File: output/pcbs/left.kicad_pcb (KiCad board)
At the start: 2 copper layers, 143.6 x 118.9 mm, 72 parts

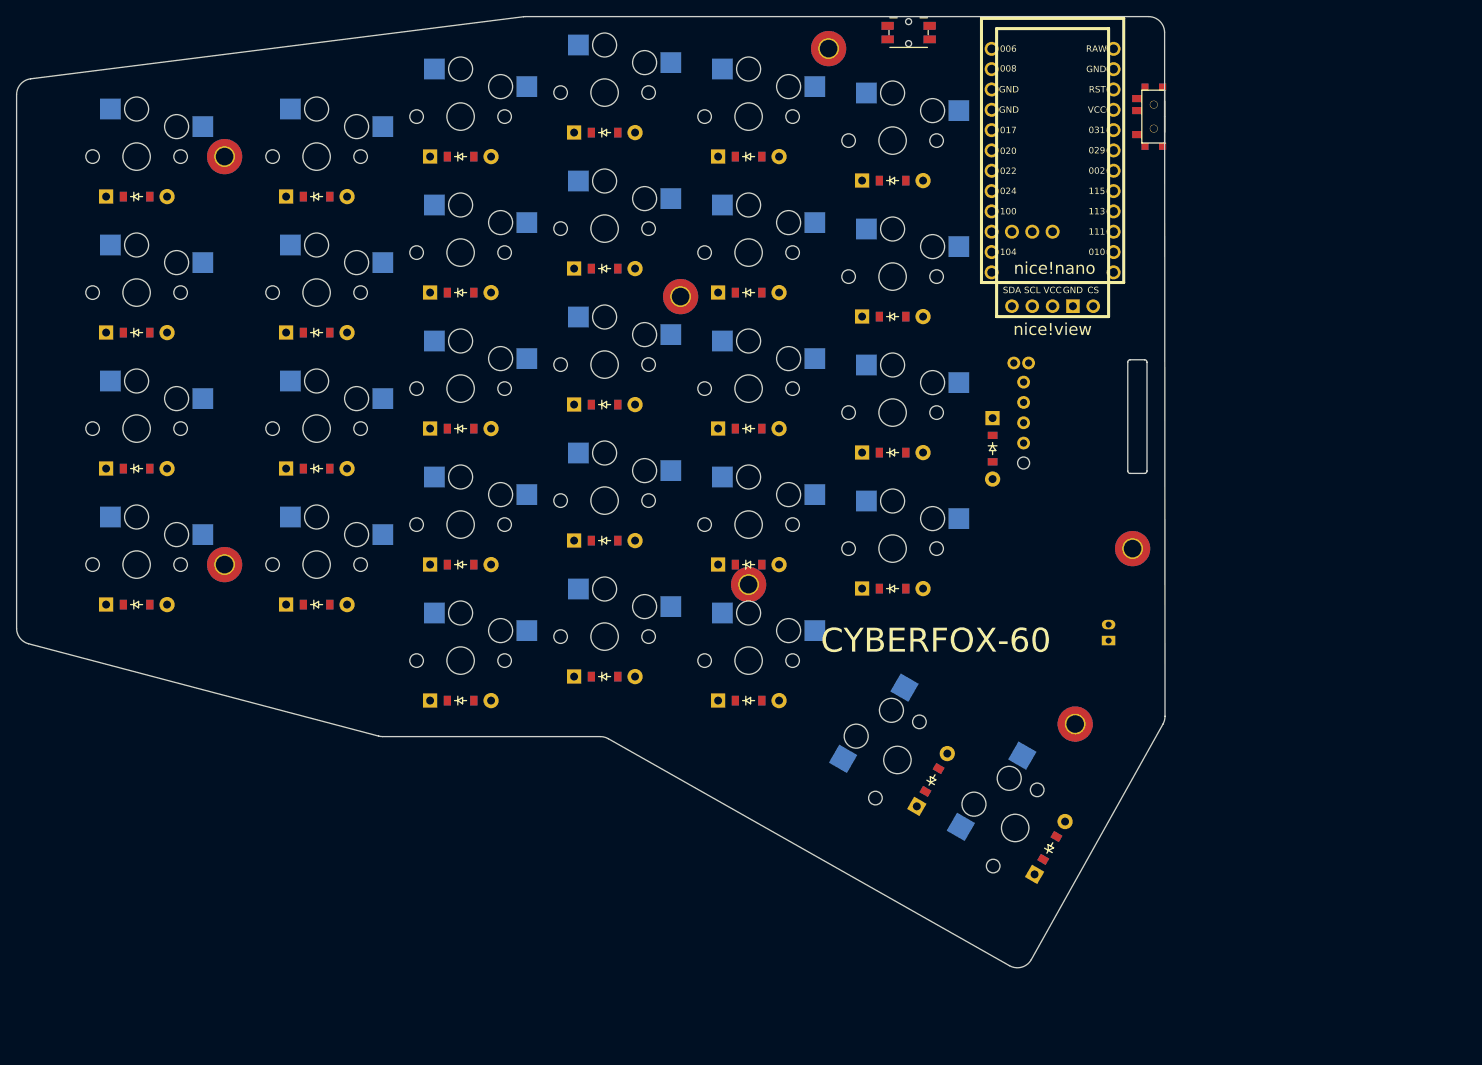
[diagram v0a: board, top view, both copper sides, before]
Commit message: Starting to trace the PCB
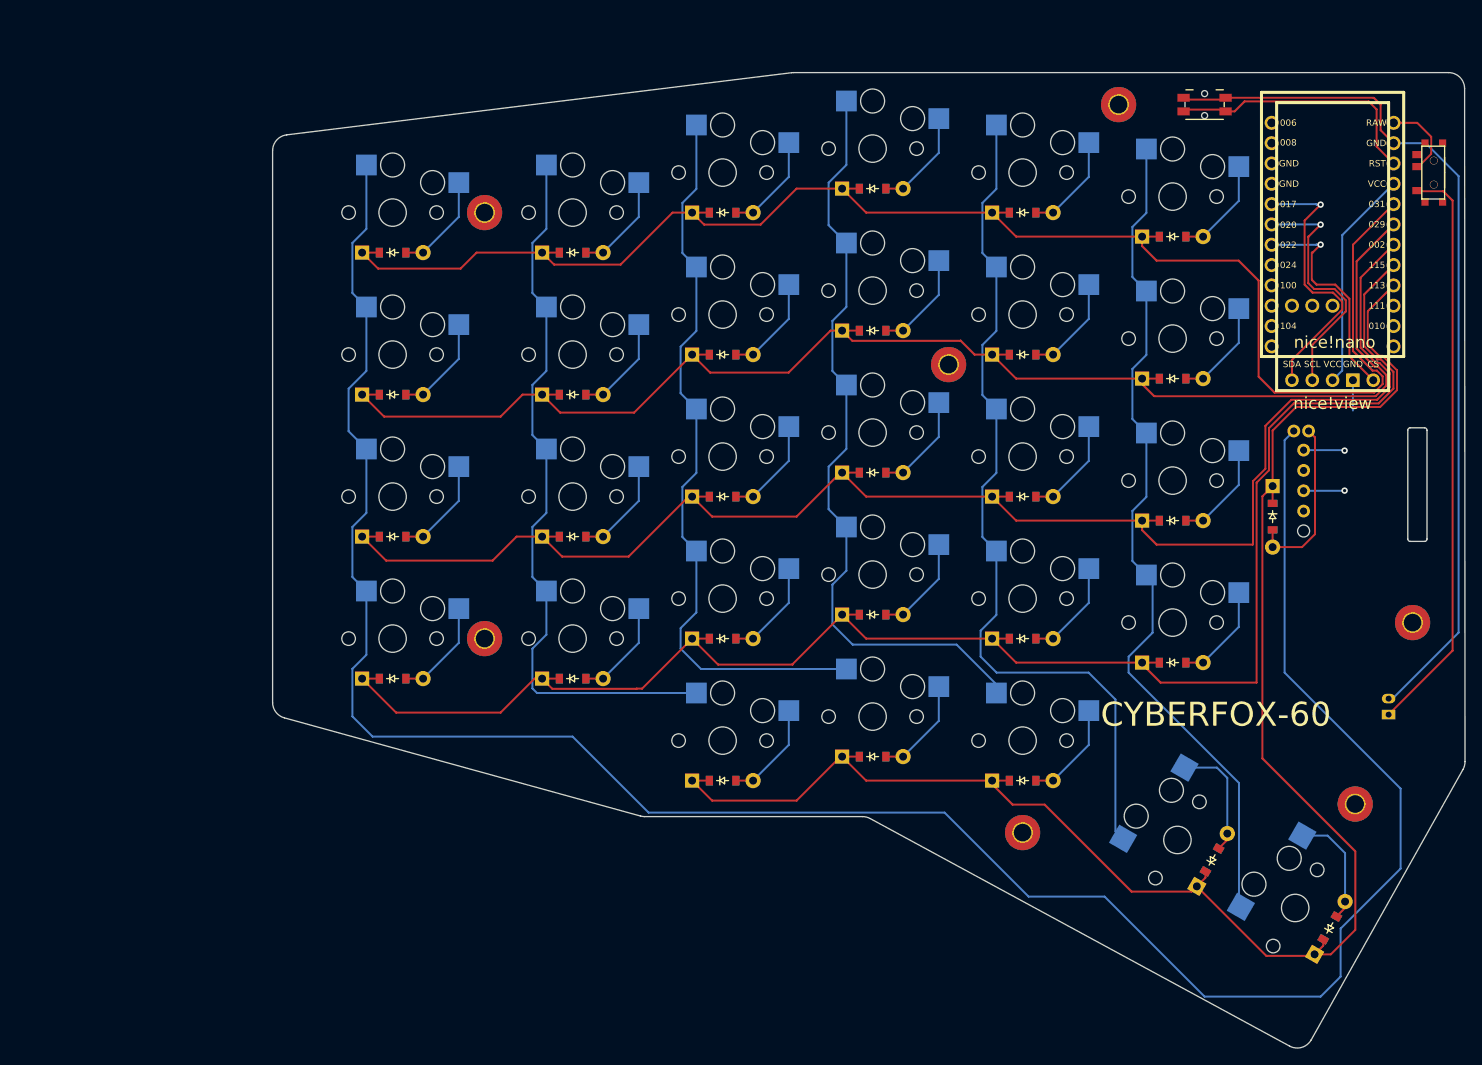
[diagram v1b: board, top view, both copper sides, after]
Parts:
- moved _8 46.2 mm to (118.8, 116.5)
- moved B1 38.1 mm to (141.5, 25.5)
- moved _4 36.9 mm to (130.8, 25.5)
- moved D28 36.4 mm to (142.4, 119.9)
- moved S28 36.4 mm to (138.1, 117.4)
- moved _2 36.4 mm to (160.3, 112.9)
- moved D29 36.4 mm to (157.2, 128.4)
- moved S29 36.4 mm to (152.8, 125.9)
- moved D24 36.2 mm to (137.5, 95.2)
- moved JST1 36.2 mm to (164.5, 100.8)
- moved MCU1 36.2 mm to (157.5, 41.8)
- moved S24 36.2 mm to (137.5, 90.2)
- moved _3 36.2 mm to (167.5, 90.2)
- moved niceView1 36.2 mm to (157.5, 61.2)
- moved D25 36.0 mm to (137.5, 77.5)
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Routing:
- net P011: track 0.00 -> 291.2 mm
- net P113: track 0.00 -> 213.5 mm
- net P115: track 0.00 -> 207.8 mm
- net P031: track 0.00 -> 193.2 mm
- net P002: track 0.00 -> 193.0 mm
- net P029: track 0.00 -> 178.5 mm
- net GND: track 0.00 -> 113.5 mm
- net P010: track 0.00 -> 108.5 mm
- net P009: track 0.00 -> 106.5 mm
- net P111: track 0.00 -> 96.0 mm
- net P106: track 0.00 -> 92.6 mm
- net P104: track 0.00 -> 91.2 mm
- net POS: track 0.00 -> 72.5 mm
- net P017: track 0.00 -> 35.0 mm, vias 0 -> 1
- net RST: track 0.00 -> 32.9 mm
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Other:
- board size 143.6 x 118.9 mm -> 149.1 x 121.9 mm
- net class Default removed
